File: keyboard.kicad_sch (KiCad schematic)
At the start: 68 parts, among them J2 TYPE-C-31-M-12, U1 ATmega32U4-A, Y1 Crystal_GND24_Small

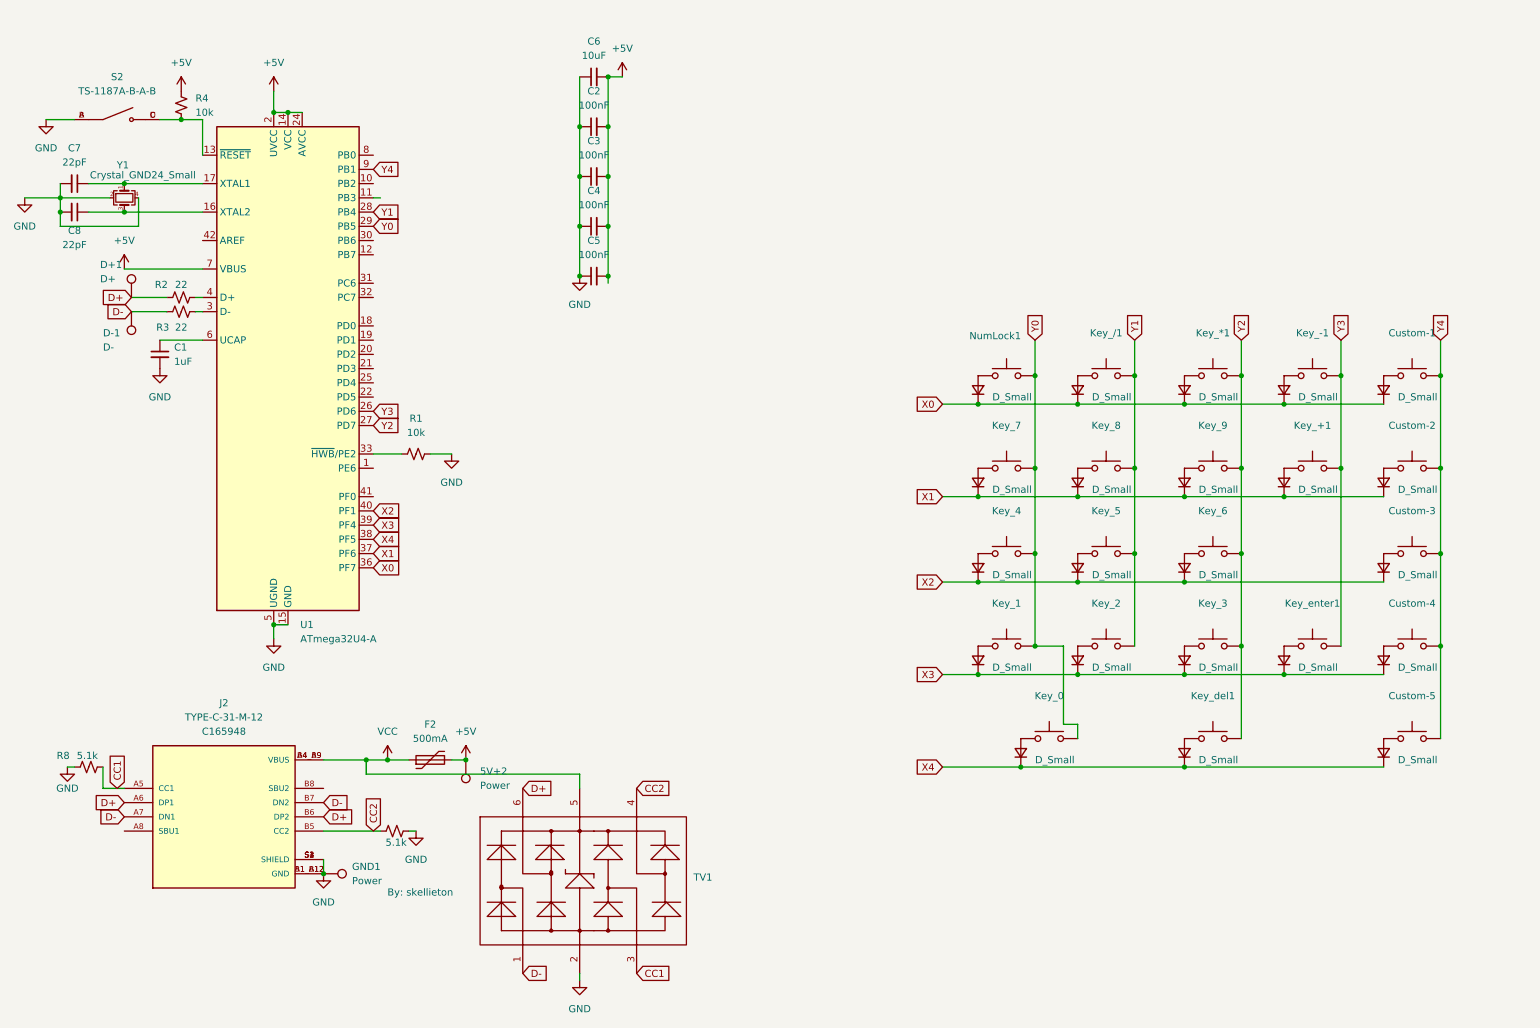
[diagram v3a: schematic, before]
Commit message: V1-with-led-schem
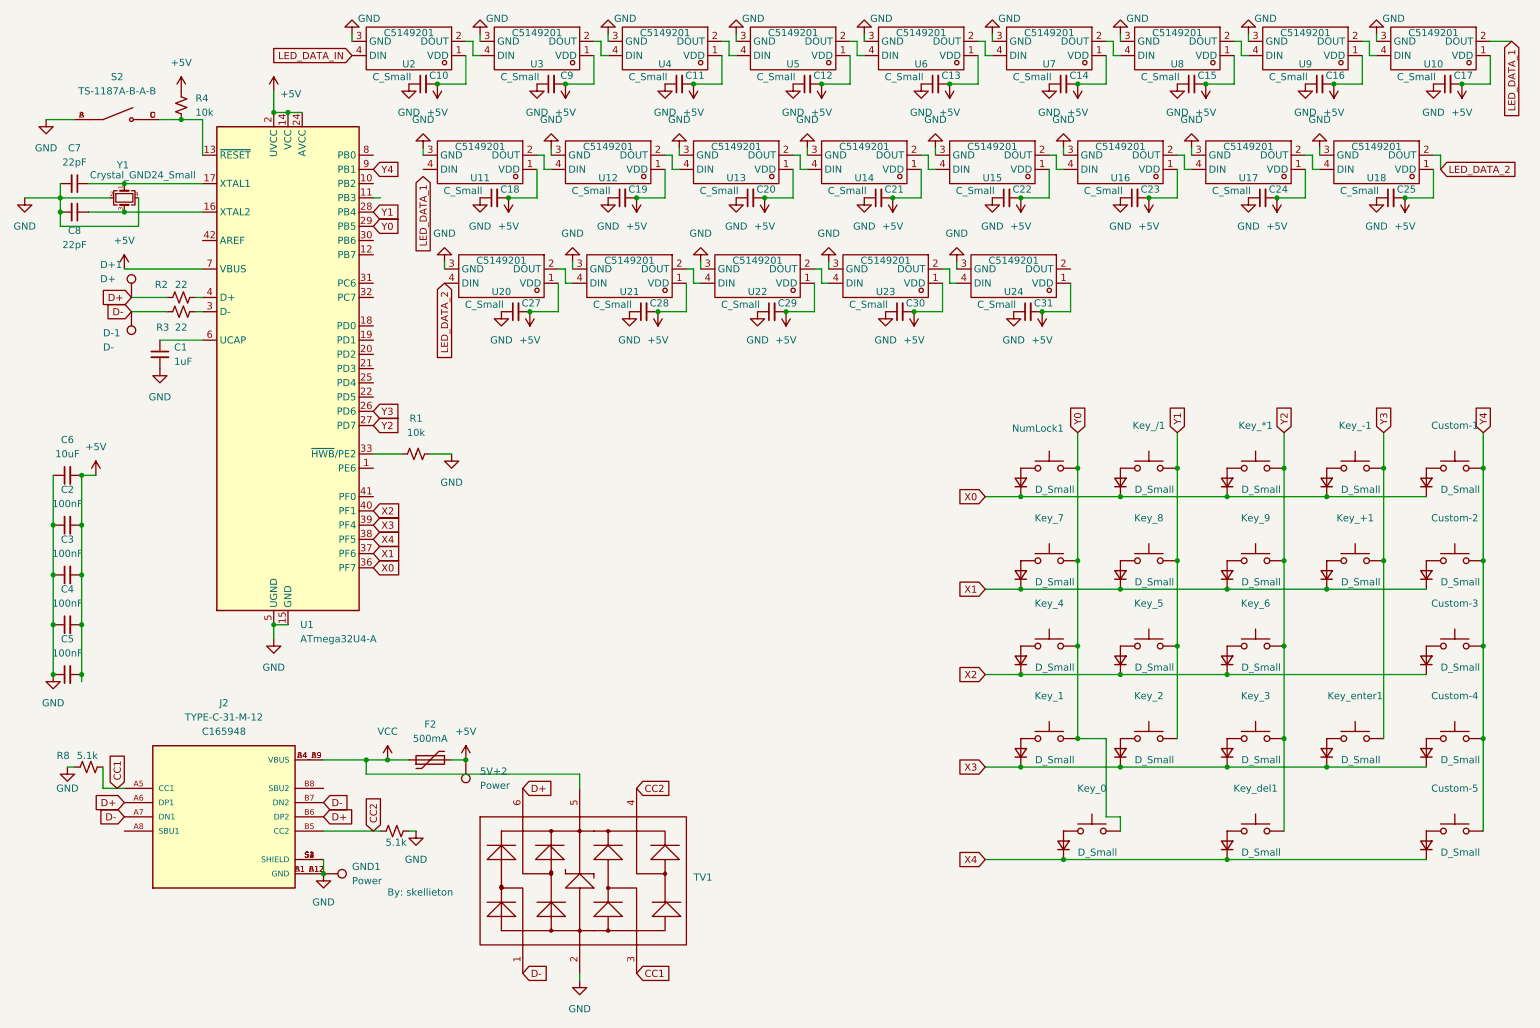
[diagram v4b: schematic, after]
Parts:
- added C10, C11, C12, C13, C14, C15, C16, C17, C18, C19, C20, C21, C22, C23, C24, C25, C27, C28, C29, C30, C31, C9: C_Small, Capacitor_SMD:C_0805_2012Metric, symbol Device:C_Small
- added U10, U11, U16, U17, U18, U20, U21, U7, U8, U9: ~, MyLiB:MX-SK-E-Right_Left, symbol MyLib:SK6812MINI-E_C5149201
- added U12, U13, U14, U15, U2, U22, U23, U24, U3, U4, U5, U6: ~, MyLiB:MX-SK-E-Left_Right, symbol MyLib:SK6812MINI-E_C5149201
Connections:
- net +5V: now also C10.2, C11.2, C12.2, C13.2, C14.2, C15.2, C16.2, C17.2, C18.2, C19.2, C20.2, C21.2, C22.2, C23.2, C24.2, C25.2, C27.2, C28.2, C29.2, C30.2, C31.2, C9.2, U10.1 (VDD), U11.1 (VDD), U12.1 (VDD), U13.1 (VDD), U14.1 (VDD), U15.1 (VDD), U16.1 (VDD), U17.1 (VDD), U18.1 (VDD), U2.1 (VDD), U20.1 (VDD), U21.1 (VDD), U22.1 (VDD), U23.1 (VDD), U24.1 (VDD), U3.1 (VDD), U4.1 (VDD), U5.1 (VDD), U6.1 (VDD), U7.1 (VDD), U8.1 (VDD), U9.1 (VDD)
- net GND: now also C10.1, C11.1, C12.1, C13.1, C14.1, C15.1, C16.1, C17.1, C18.1, C19.1, C20.1, C21.1, C22.1, C23.1, C24.1, C25.1, C27.1, C28.1, C29.1, C30.1, C31.1, C9.1, U10.3 (GND), U11.3 (GND), U12.3 (GND), U13.3 (GND), U14.3 (GND), U15.3 (GND), U16.3 (GND), U17.3 (GND), U18.3 (GND), U2.3 (GND), U20.3 (GND), U21.3 (GND), U22.3 (GND), U23.3 (GND), U24.3 (GND), U3.3 (GND), U4.3 (GND), U5.3 (GND), U6.3 (GND), U7.3 (GND), U8.3 (GND), U9.3 (GND)
- new net: U12.2 (DOUT), U13.4 (DIN)
- new net: U11.2 (DOUT), U12.4 (DIN)
- new net: U22.2 (DOUT), U23.4 (DIN)
- new net: U21.2 (DOUT), U22.4 (DIN)
- new net: U20.2 (DOUT), U21.4 (DIN)
- new net: U15.2 (DOUT), U16.4 (DIN)
- new net: U14.2 (DOUT), U15.4 (DIN)
- new net: U16.2 (DOUT), U17.4 (DIN)
- new net: U3.2 (DOUT), U4.4 (DIN)
- new net: U2.2 (DOUT), U3.4 (DIN)
- new net: U7.2 (DOUT), U8.4 (DIN)
- new net: U6.2 (DOUT), U7.4 (DIN)
- new net: U17.2 (DOUT), U18.4 (DIN)
- new net: U10.4 (DIN), U9.2 (DOUT)
- new net: U8.2 (DOUT), U9.4 (DIN)
- new net: U23.2 (DOUT), U24.4 (DIN)
- new net: U13.2 (DOUT), U14.4 (DIN)
- new net: U5.2 (DOUT), U6.4 (DIN)
- new net: U4.2 (DOUT), U5.4 (DIN)
- new net LED_DATA_1: U10.2 (DOUT)
- new net LED_DATA_2: U18.2 (DOUT), U20.4 (DIN)
- new net LED_DATA_IN: U2.4 (DIN)
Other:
- moved on the sheet: C2, C3, C4, C5, C6, Custom-1, Custom-2, Custom-3, Custom-4, Custom-5, Key_*1, Key_+1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
